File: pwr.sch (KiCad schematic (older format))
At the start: 55 parts, among them U1 FT601, U10 MIC94310, U11 PAM2305, U4 ECP5, U6 PAM2305, U7 NCP186, U8 MIC94310, U9 MIC94310, X2 CONN_01X08

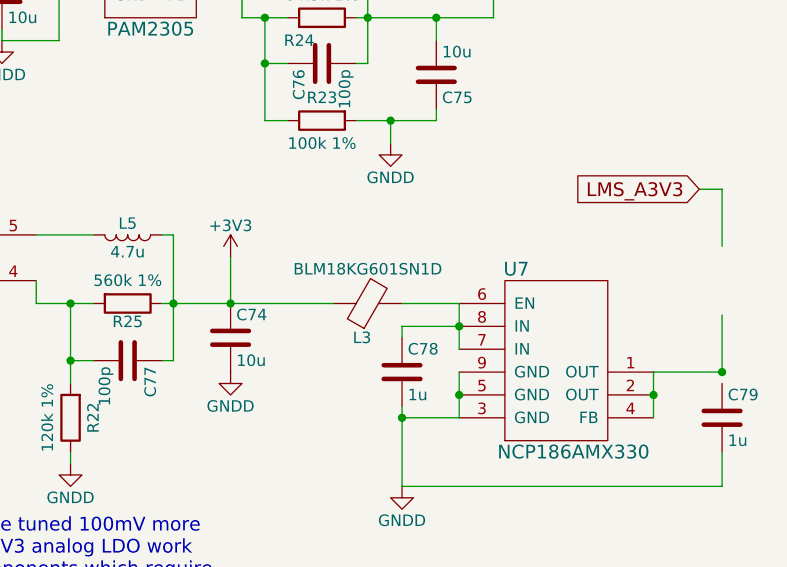
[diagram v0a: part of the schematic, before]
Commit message: Right before switching to full RPi
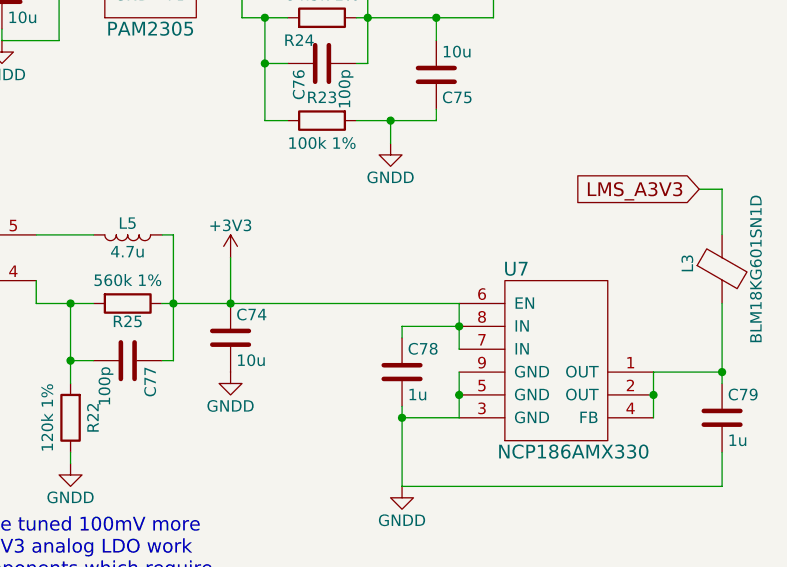
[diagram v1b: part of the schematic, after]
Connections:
- net +3V3: now also C78.1, U7.6 (EN), U7.7 (IN), U7.8 (IN); no longer L3.1
- net LMS_A3V3: now also L3.1
- net at U7.1 (OUT), U7.2 (OUT), U7.4 (FB): now also C79.1, L3.2
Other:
- moved on the sheet: L3
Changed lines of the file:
@@
 L Ferrite_Bead L3
 U 1 1 58C779A8
-P 9250 5200
-F 0 "L3" V 9100 5225 50  0000 C CNN
-F 1 "BLM18KG601SN1D" V 9400 5200 50  0000 C CNN
-F 2 "Capacitors_SMD:C_0805" V 9180 5200 50  0001 C CNN
-F 3 "" H 9250 5200 50  0000 C CNN
-	1    9250 5200
-	0    -1   -1   0
+P 10800 5050
+F 0 "L3" V 10650 5075 50  0000 C CNN
+F 1 "BLM18KG601SN1D" V 10950 5050 50  0000 C CNN
+F 2 "Capacitors_SMD:C_0805" V 10730 5050 50  0001 C CNN
+F 3 "" H 10800 5050 50  0000 C CNN
+	1    10800 5050
+	1    0    0    -1
 $EndComp
-Wire Wire Line
-	10800 5500 10800 5250
-Wire Wire Line
-	10800 4950 10800 4700
 Text GLabel 3600 6850 0    60   Input ~ 0
 LMS_A3V3
@@
 $EndComp
 Wire Wire Line
-	9400 5200 9650 5200
-Wire Wire Line
-	8350 5200 9100 5200
+	8350 5200 9650 5200
 Wire Wire Line
 	8650 5000 8650 5200
+Wire Wire Line
+	10800 5200 10800 5550
+Wire Wire Line
+	10800 4700 10800 4900
 $EndSCHEMATC
